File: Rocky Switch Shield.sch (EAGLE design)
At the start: 33 parts

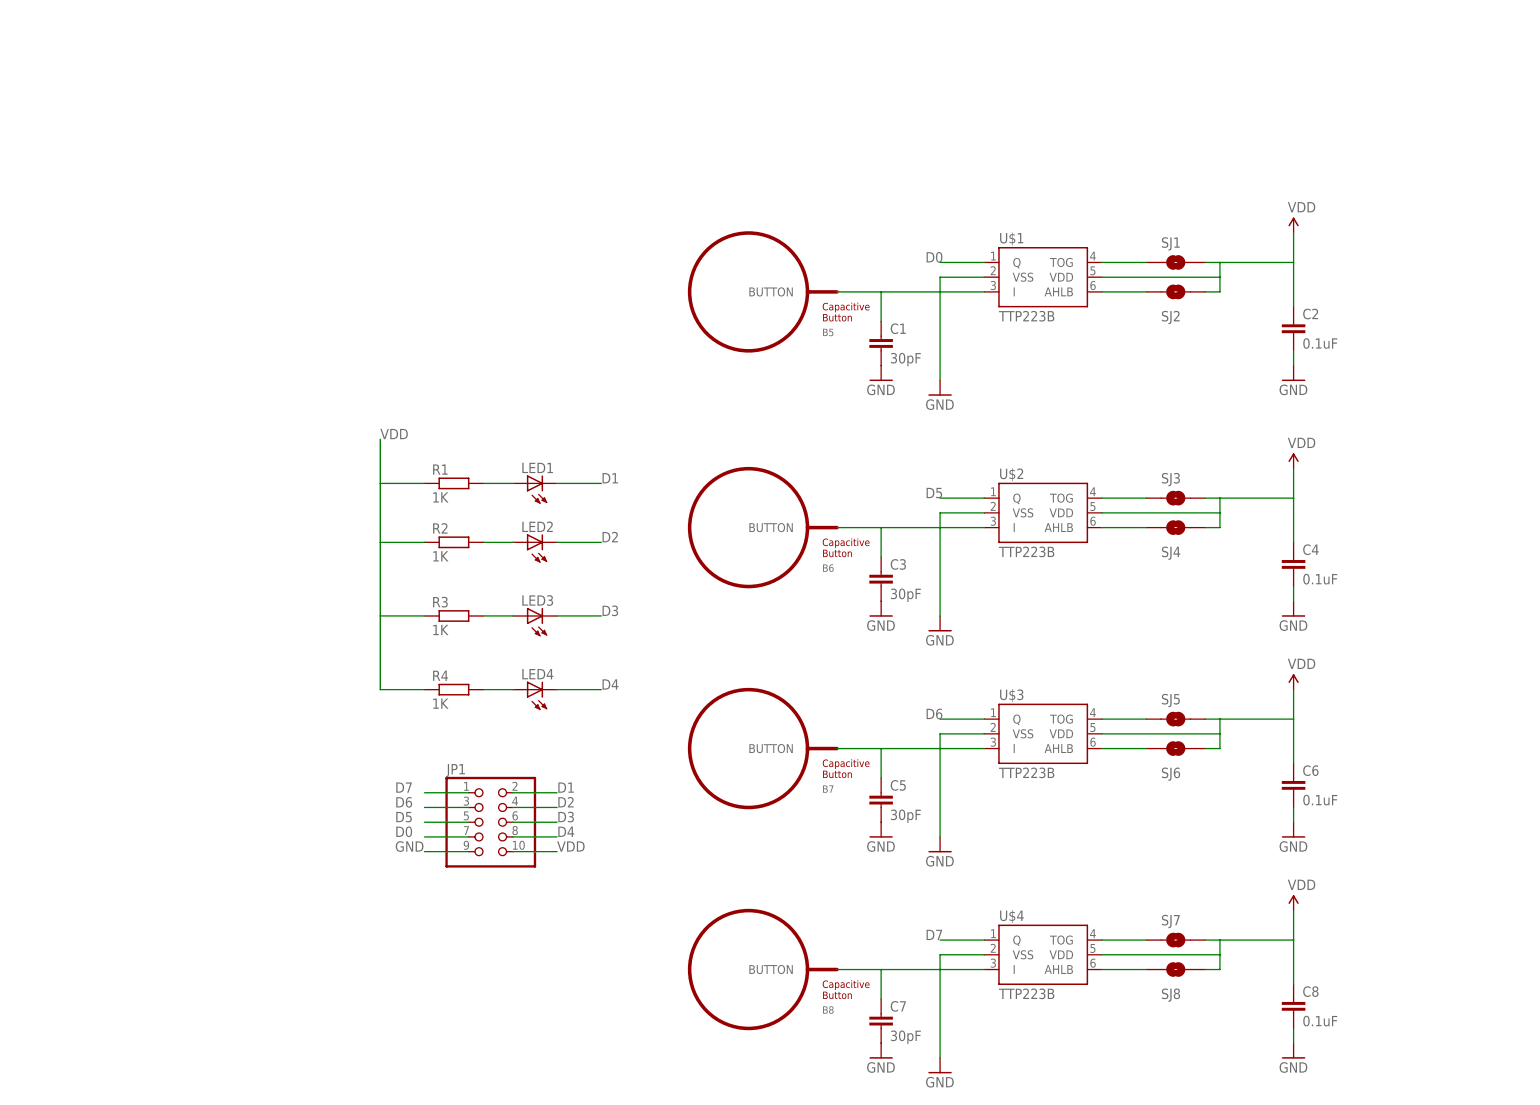
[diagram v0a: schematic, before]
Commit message: Update board design to version 0.2
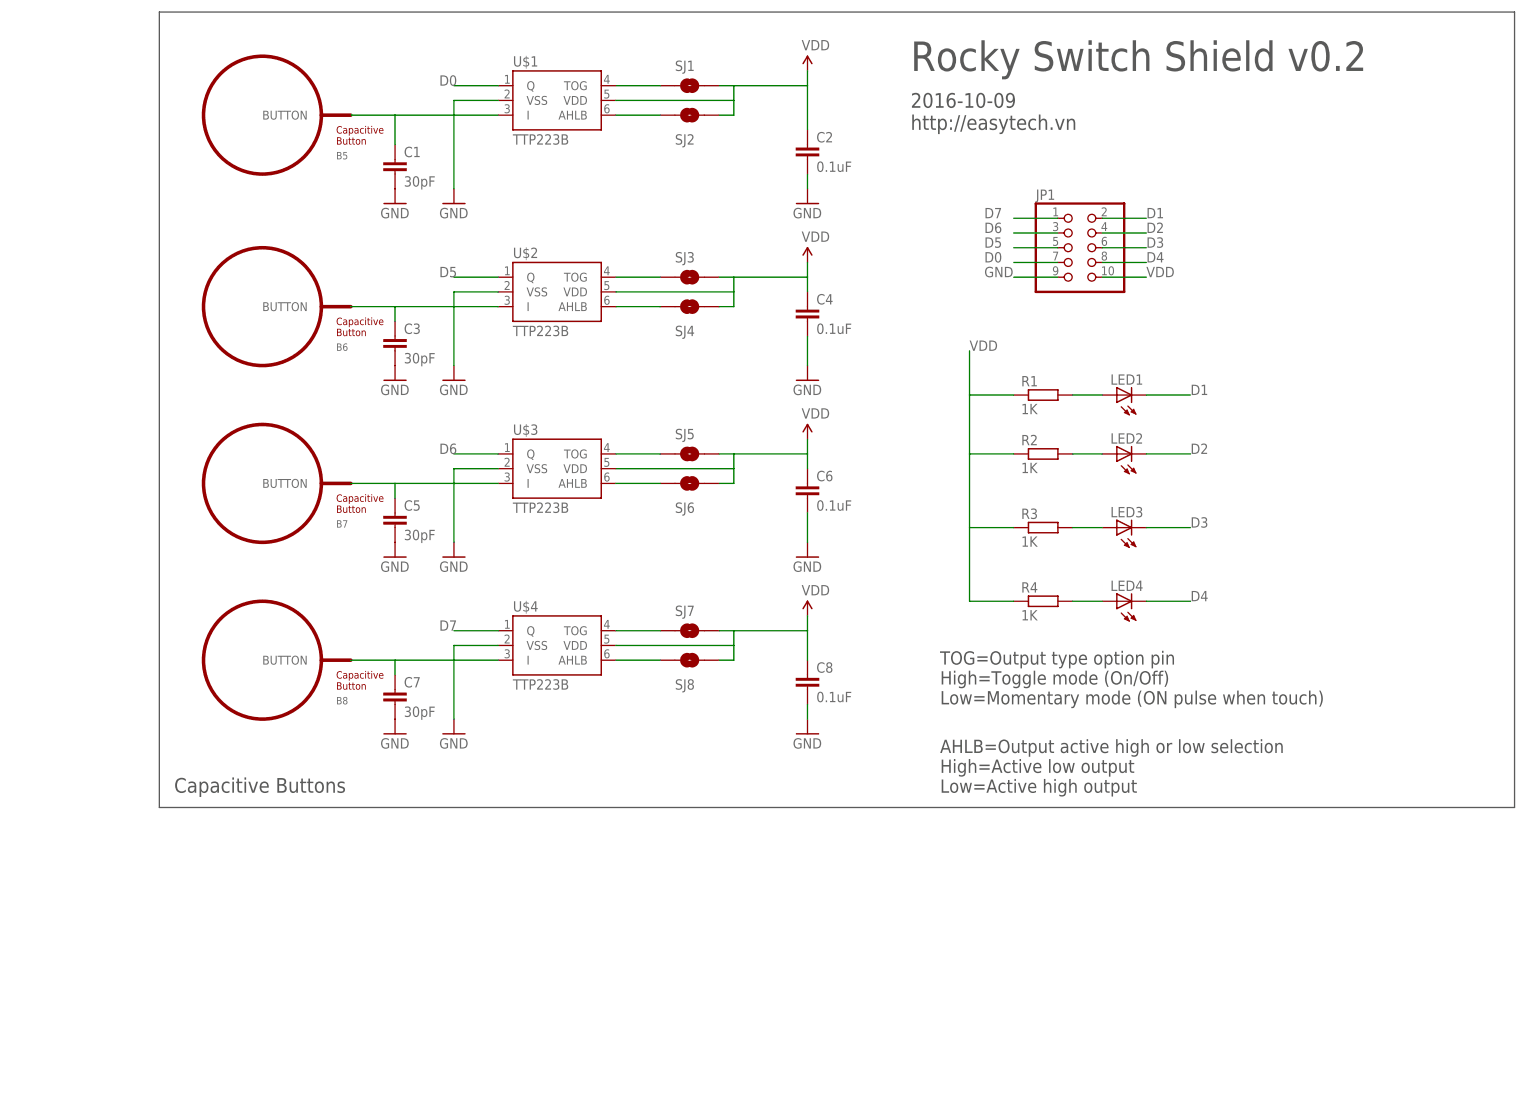
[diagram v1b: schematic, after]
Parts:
- LED1, LED2, LED3, LED4: device adafruit:LED3MM -> adafruit:LEDCHIP-LED0805
- SJ1, SJ3, SJ5, SJ7: value JUMPER-PAD-2-NOYES_SILK -> AHLB
- SJ2, SJ4, SJ6, SJ8: value JUMPER-PAD-2-NOYES_SILK -> TOG
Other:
- note added: "2016-10-09 http://easytech.vn"
- note added: "AHLB=Output active high or low selection High=Active low output Low=Active high output"
- note added: "Capacitive Buttons"
- note added: "Rocky Switch Shield v0.2"
- note added: "TOG=Output type option pin High=Toggle mode (On/Off) Low=Momentary mode (ON pulse when touch)"
- moved on the sheet: B5, B6, B7, B8, C1, C2, C3, C4, C5, C6, C7, C8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

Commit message: Update design to version 0.3
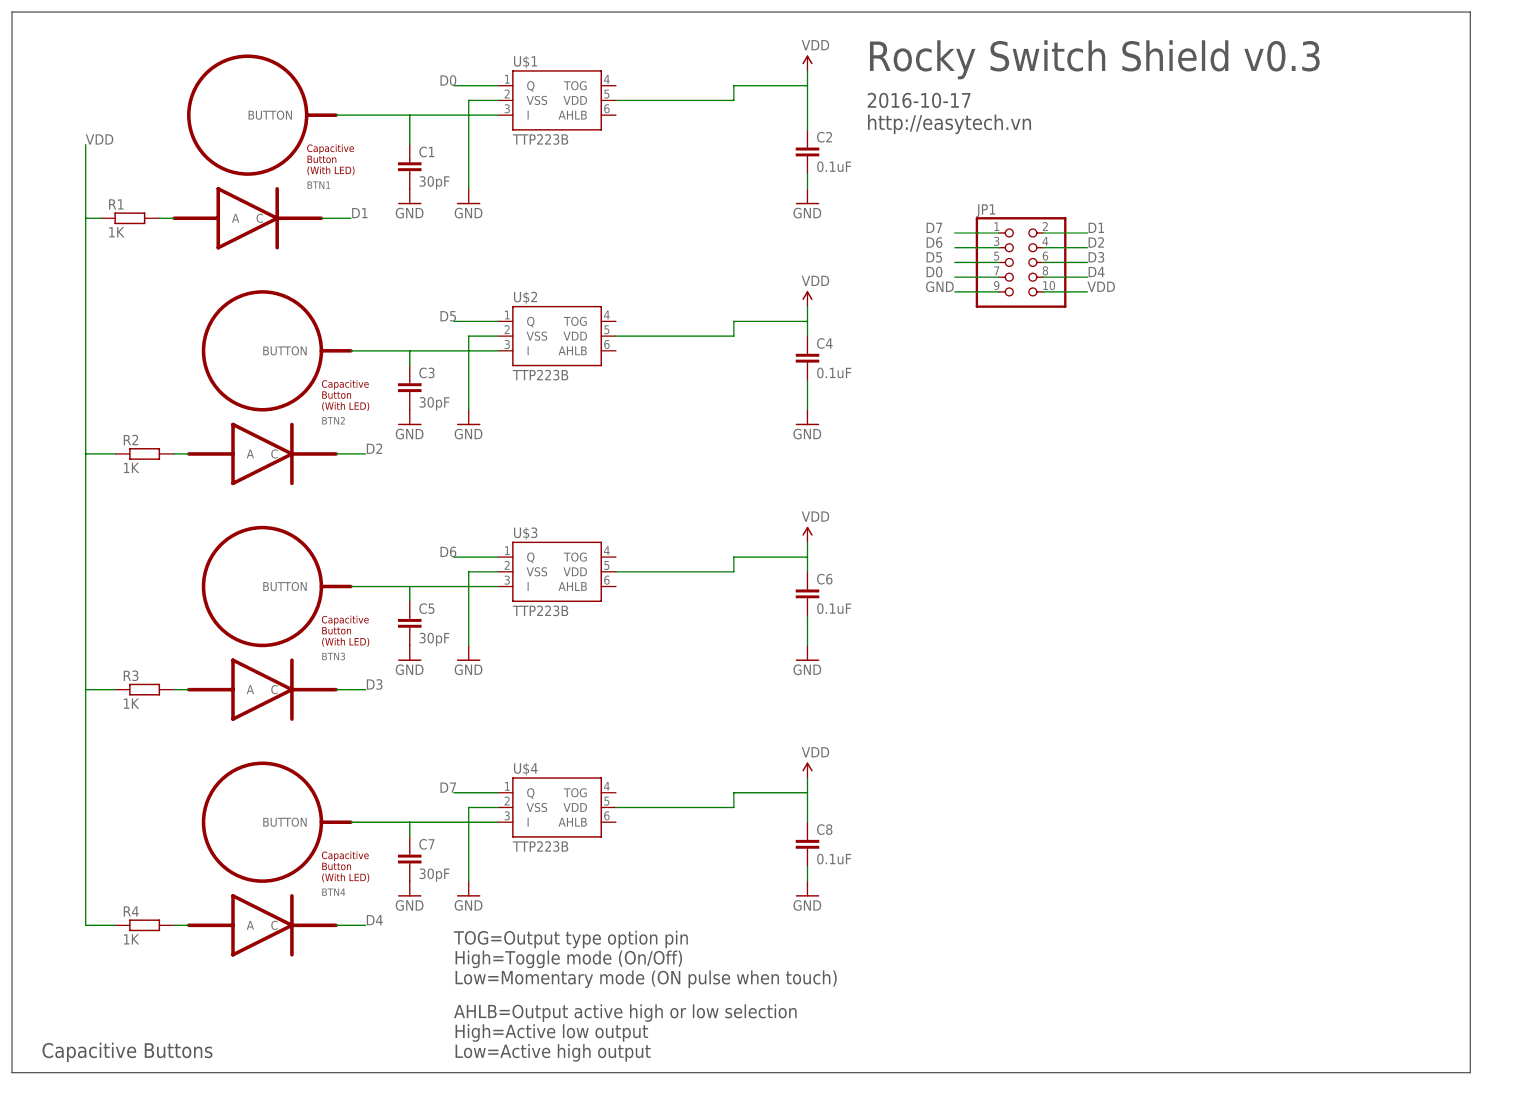
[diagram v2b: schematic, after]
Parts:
- removed B5, B6, B7, B8: (no value), PatternAgents-TouchWidgets:BUTTON_PASSIVE12MM
- removed LED1, LED2, LED3, LED4: (no value), adafruit:LEDCHIP-LED0805
- removed SJ1, SJ3, SJ5, SJ7: AHLB, SparkFun-Passives:JUMPER-PAD-2-NOYES_SILK
- removed SJ2, SJ4, SJ6, SJ8: TOG, SparkFun-Passives:JUMPER-PAD-2-NOYES_SILK
- added BTN1, BTN2, BTN3, BTN4: BUTTON_PASSIVE_LED, My Eagle Lib:BUTTON_PASSIVE_LED
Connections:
- removed net N$1: SJ1.1, U$1.TOG
- removed net N$11: SJ5.1, U$3.TOG
- removed net N$12: SJ6.1, U$3.AHLB
- removed net N$15: SJ7.1, U$4.TOG
- removed net N$16: SJ8.1, U$4.AHLB
- removed net N$3: LED1.A, R1.2
- removed net N$4: LED2.A, R2.2
- removed net N$5: SJ2.1, U$1.AHLB
- removed net N$6: LED3.A, R3.2
- removed net N$7: SJ3.1, U$2.TOG
- removed net N$8: SJ4.1, U$2.AHLB
- removed net N$9: LED4.A, R4.2
- new net N$10: BTN1.A, R1.2
- new net N$13: BTN2.A, R2.2
- new net N$14: BTN3.A, R3.2
- new net N$17: BTN4.A, R4.2
- net D1: now also BTN1.C; no longer LED1.C
- net D2: now also BTN2.C; no longer LED2.C
- net D3: now also BTN3.C; no longer LED3.C
- net D4: now also BTN4.C; no longer LED4.C
- net I1: now also BTN1.BUTTON; no longer B5.BUTTON
- net I2: now also BTN2.BUTTON; no longer B6.BUTTON
- net I3: now also BTN3.BUTTON; no longer B7.BUTTON
- net I4: now also BTN4.BUTTON; no longer B8.BUTTON
- net VDD: no longer SJ1.2, SJ2.2, SJ3.2, SJ4.2, SJ5.2, SJ6.2, SJ7.2, SJ8.2
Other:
- note added: "2016-10-17 http://easytech.vn"
- note added: "Rocky Switch Shield v0.3"
- note removed: "2016-10-09 http://easytech.vn"
- note removed: "Rocky Switch Shield v0.2"
- moved on the sheet: C1, C3, C4, C5, C6, C7, C8, JP1, R1, R2, R3, R4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
